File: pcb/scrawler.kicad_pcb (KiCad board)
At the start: 2 copper layers, 54 parts, among them SW1 switch, SW10 switch, SW11 switch, SW12 switch, SW13 switch, SW14 switch, SW15 switch, SW16 switch, SW17 switch, SW18 switch, SW19 switch, SW2 switch, SW20 switch, SW21 switch, SW22 switch, SW23 switch, SW3 switch, SW4 switch, SW5 switch, SW6 switch, SW7 switch, SW8 switch, SW9 switch, U1 TRRS, U2 ProMicro

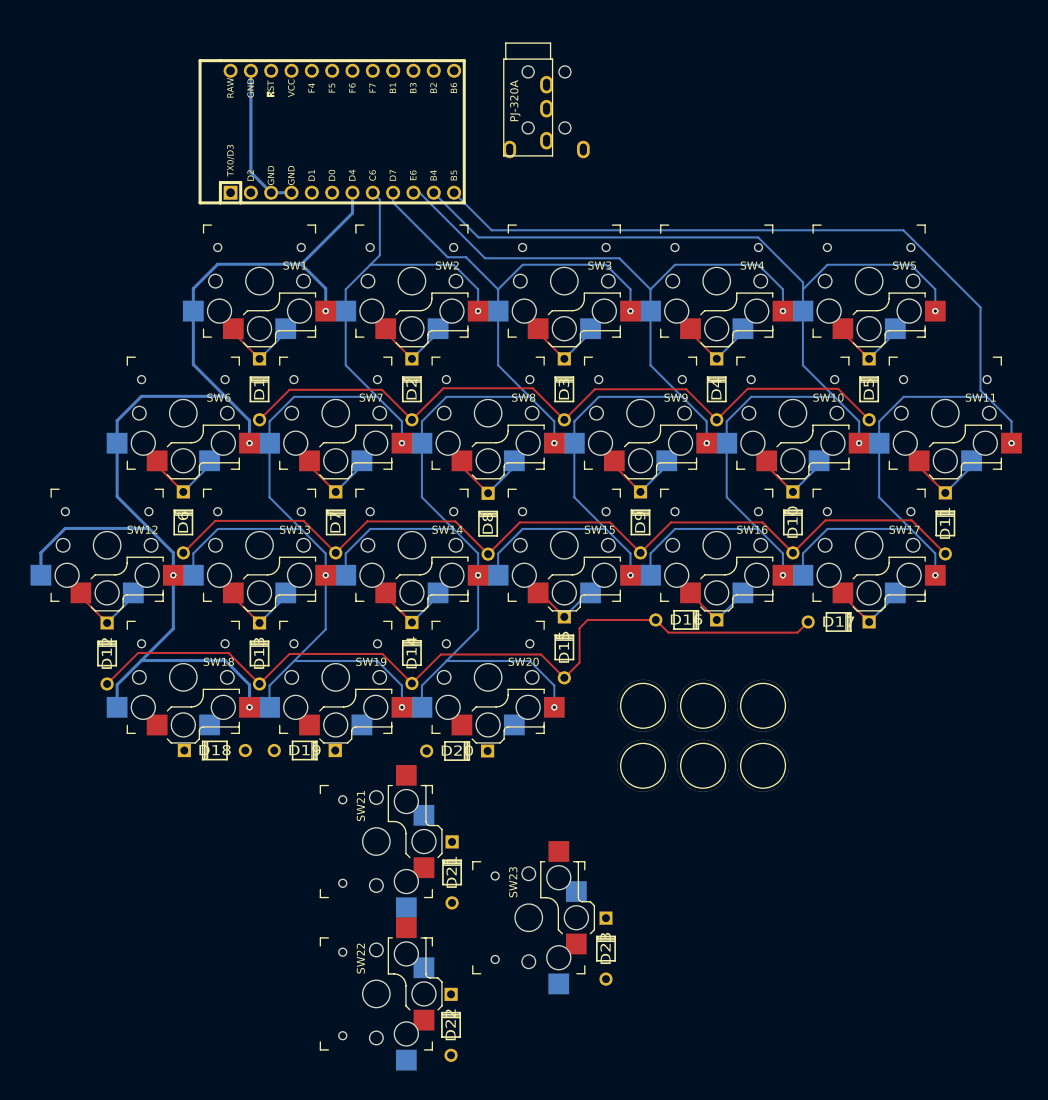
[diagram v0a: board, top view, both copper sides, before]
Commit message: finished routing
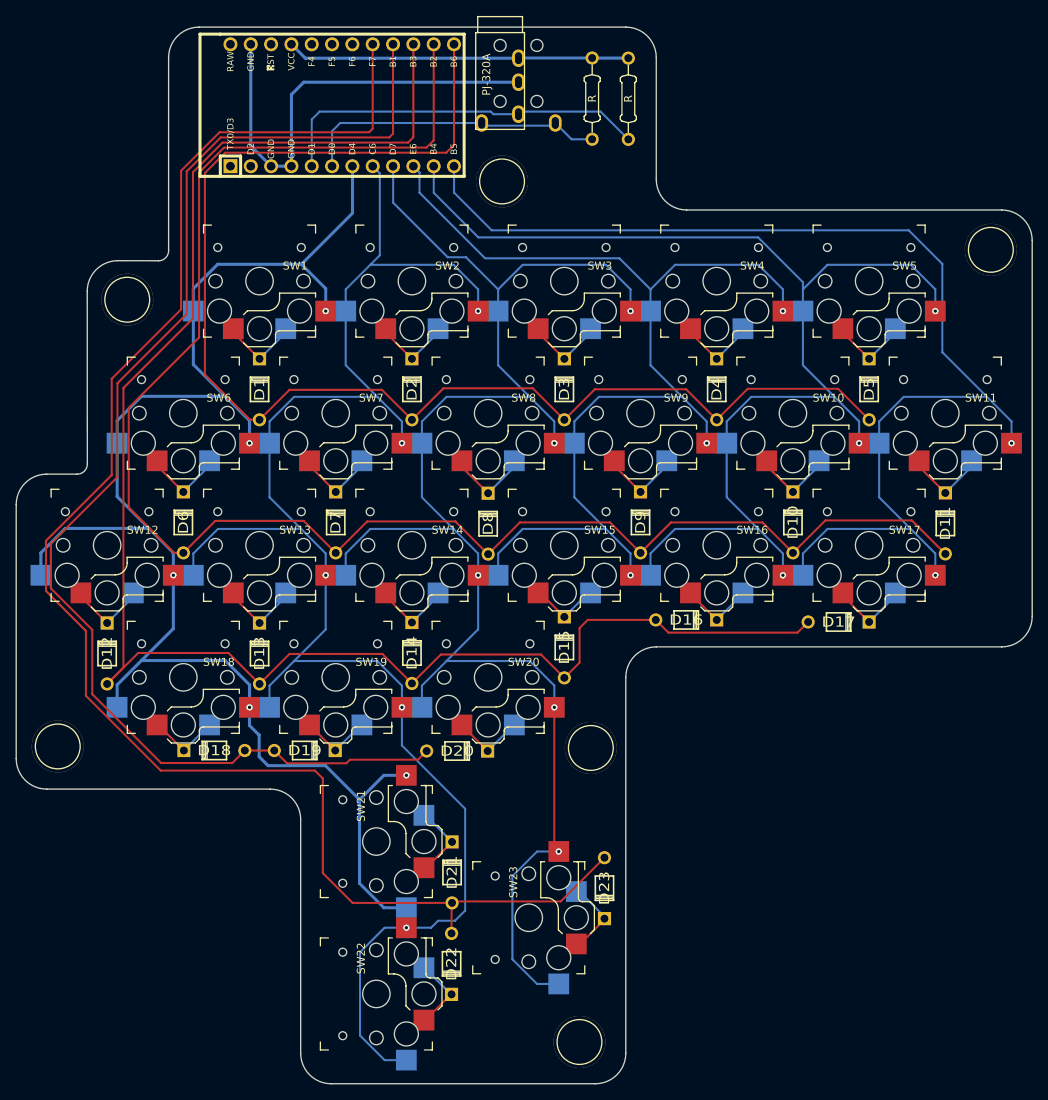
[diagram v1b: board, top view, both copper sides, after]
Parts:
- added R1: R, Keebio-Parts:Resistor, F.Cu at (165.4, 33.1)
- added R2: R, Keebio-Parts:Resistor, F.Cu at (160.9, 33.1)
- moved H3 88.1 mm to (102.8, 58.2)
- moved H4 80.7 mm to (94.1, 114.0)
- moved H5 73.2 mm to (149.6, 43.4)
- moved H6 70.5 mm to (210.7, 52.0)
- moved H2 35.4 mm to (159.3, 151.0)
- moved H1 8.39 mm to (160.7, 114.2)
- moved D22 7.62 mm to (143.3, 141.2), turned to 270 degrees
- moved D23 7.56 mm to (162.4, 131.8), turned to 270 degrees
- moved U1 4.82 mm to (151.7, 24.8)
- moved U2 3.31 mm to (129.7, 33.9)
- moved D18 0.06 mm to (113.7, 114.6)
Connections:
- U1 pad 1: VCC -> SCL
- U1 pad 3: SCL -> GND
- U1 pad 4: GND -> VCC
- U2 pad 13: ROW4 -> ROW0
- U2 pad 14: ROW3 -> ROW1
- U2 pad 16: ROW1 -> ROW3
- U2 pad 17: ROW0 -> ROW4
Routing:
- net ROW4: track 0.00 -> 200.0 mm
- net ROW3: track 0.00 -> 160.7 mm
- net ROW2: track 103.4 -> 212.8 mm
- net ROW1: track 111.7 -> 209.4 mm
- net ROW0: track 88.9 -> 168.5 mm
- net COL1: track 145.1 -> 209.8 mm, vias 4 -> 5
- net COL0: track 147.3 -> 196.7 mm, vias 4 -> 5
- net SDA: track 0.00 -> 47.5 mm
- net COL2: track 154.1 -> 200.2 mm, vias 4 -> 5
- net VCC: track 0.00 -> 42.8 mm
- net SCL: track 0.00 -> 38.4 mm
- net GND: track 18.8 -> 56.8 mm
- net Net-(D19-Pad2): track 0.00 -> 10.2 mm
- net Net-(D23-Pad2): track 0.00 -> 10.1 mm
- net Net-(D21-Pad2): track 0.00 -> 9.74 mm
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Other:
- board outline added: 127 x 132.1 mm
